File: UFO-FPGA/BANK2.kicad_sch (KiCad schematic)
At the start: 3 parts, among them U4 ICE40HX4K-TQ144

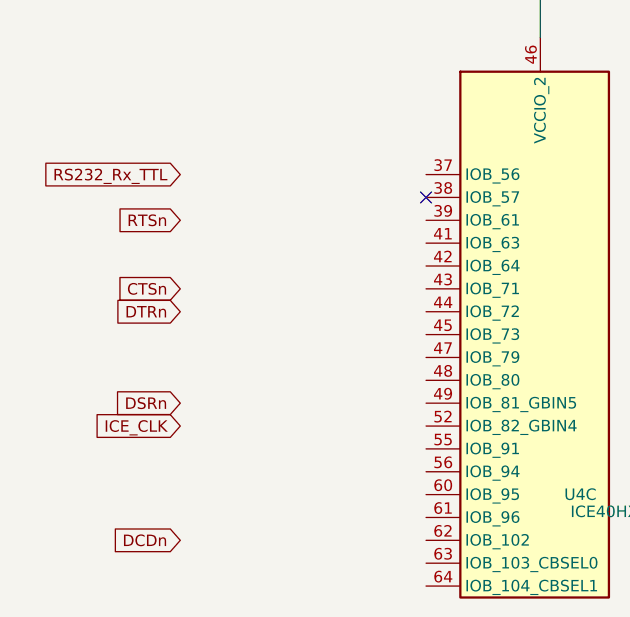
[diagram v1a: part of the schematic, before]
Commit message: pcb
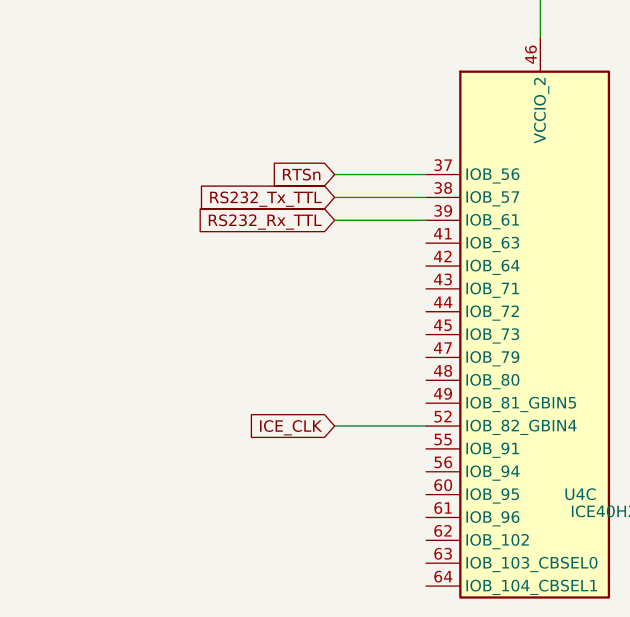
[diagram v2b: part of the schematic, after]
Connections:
- net ICE_CLK: now also U4.52 (IOB_82_GBIN4)
- net RS232_Rx_TTL: now also U4.39 (IOB_61)
- net RTSn: now also U4.37 (IOB_56)
- net RS232_Tx_TTL: now reaches U4.38 (IOB_57)
- no-connect marks 1 -> 0
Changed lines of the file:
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@@
   (junction (at 163.83 52.07) (diameter 0) (color 0 0 0 0)
   )
-  (no_connect (at 113.665 82.55))
+  (wire (pts (xy 103.505 82.55) (xy 113.665 82.55))
+    (stroke (width 0) (type default))
+  )
   (wire (pts (xy 152.4 59.69) (xy 163.83 59.69))
     (stroke (width 0) (type default))
@@
     (stroke (width 0) (type default))
   )
+  (wire (pts (xy 103.505 80.01) (xy 113.665 80.01))
+    (stroke (width 0) (type default))
+  )
+  (wire (pts (xy 103.505 107.95) (xy 113.665 107.95))
+    (stroke (width 0) (type default))
+  )
+  (wire (pts (xy 103.505 85.09) (xy 113.665 85.09))
+    (stroke (width 0) (type default))
+  )
   (wire (pts (xy 192.405 41.91) (xy 192.405 52.07))
     (stroke (width 0) (type default))
@@
     (effects (font (size 1.27 1.27)) (justify left bottom))
   )
-  (global_label "CTSn" (shape input) (at 86.36 92.71 180) (fields_autoplaced)
+  (global_label "RS232_Tx_TTL" (shape input) (at 103.505 82.55 180) (fields_autoplaced)
     (effects (font (size 1.27 1.27)) (justify right))
-    (property "Intersheetrefs" "${INTERSHEET_REFS}" (at 78.8581 92.71 0)
+    (property "Intersheetrefs" "${INTERSHEET_REFS}" (at 87.597 82.55 0)
       (effects (font (size 1.27 1.27)) (justify right) hide)
     )
   )
-  (global_label "DCDn" (shape input) (at 86.36 120.65 180) (fields_autoplaced)
+  (global_label "RS232_Rx_TTL" (shape input) (at 103.505 85.09 180) (fields_autoplaced)
     (effects (font (size 1.27 1.27)) (justify right))
-    (property "Intersheetrefs" "${INTERSHEET_REFS}" (at 78.4952 120.65 0)
+    (property "Intersheetrefs" "${INTERSHEET_REFS}" (at 87.2946 85.09 0)
       (effects (font (size 1.27 1.27)) (justify right) hide)
     )
   )
-  (global_label "DTRn" (shape input) (at 86.36 95.25 180) (fields_autoplaced)
+  (global_label "RTSn" (shape input) (at 103.505 80.01 180) (fields_autoplaced)
     (effects (font (size 1.27 1.27)) (justify right))
-    (property "Intersheetrefs" "${INTERSHEET_REFS}" (at 78.7976 95.25 0)
+    (property "Intersheetrefs" "${INTERSHEET_REFS}" (at 96.0031 80.01 0)
       (effects (font (size 1.27 1.27)) (justify right) hide)
     )
   )
-  (global_label "RS232_Rx_TTL" (shape input) (at 86.36 80.01 180) (fields_autoplaced)
+  (global_label "ICE_CLK" (shape input) (at 103.505 107.95 180) (fields_autoplaced)
     (effects (font (size 1.27 1.27)) (justify right))
-    (property "Intersheetrefs" "${INTERSHEET_REFS}" (at 70.1496 80.01 0)
+    (property "Intersheetrefs" "${INTERSHEET_REFS}" (at 93.0397 107.95 0)
       (effects (font (size 1.27 1.27)) (justify right) hide)
     )
-  )
-  (global_label "DSRn" (shape input) (at 86.36 105.41 180) (fields_autoplaced)
-    (effects (font (size 1.27 1.27)) (justify right))
-    (property "Intersheetrefs" "${INTERSHEET_REFS}" (at 78.5557 105.41 0)
-      (effects (font (size 1.27 1.27)) (justify right) hide)
-    )
-  )
-  (global_label "RTSn" (shape input) (at 86.36 85.09 180) (fields_autoplaced)
-    (effects (font (size 1.27 1.27)) (justify right))
-    (property "Intersheetrefs" "${INTERSHEET_REFS}" (at 78.8581 85.09 0)
-      (effects (font (size 1.27 1.27)) (justify right) hide)
-    )
-  )
-  (global_label "ICE_CLK" (shape input) (at 86.36 107.95 180) (fields_autoplaced)
-    (effects (font (size 1.27 1.27)) (justify right))
-    (property "Intersheetrefs" "${INTERSHEET_REFS}" (at 75.8947 107.95 0)
-      (effects (font (size 1.27 1.27)) (justify right) hide)
-    )
